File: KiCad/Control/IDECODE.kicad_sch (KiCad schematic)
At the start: 17 parts, among them U10 74HCT32, U12 28C16, U13 28C16, U14 74HCT163, U15 74HCT00, U16 74HCT32, U17 74HCT04, U2 74HCT04, U23 74HCT04, U28 74HCT08, U9 74HCT08

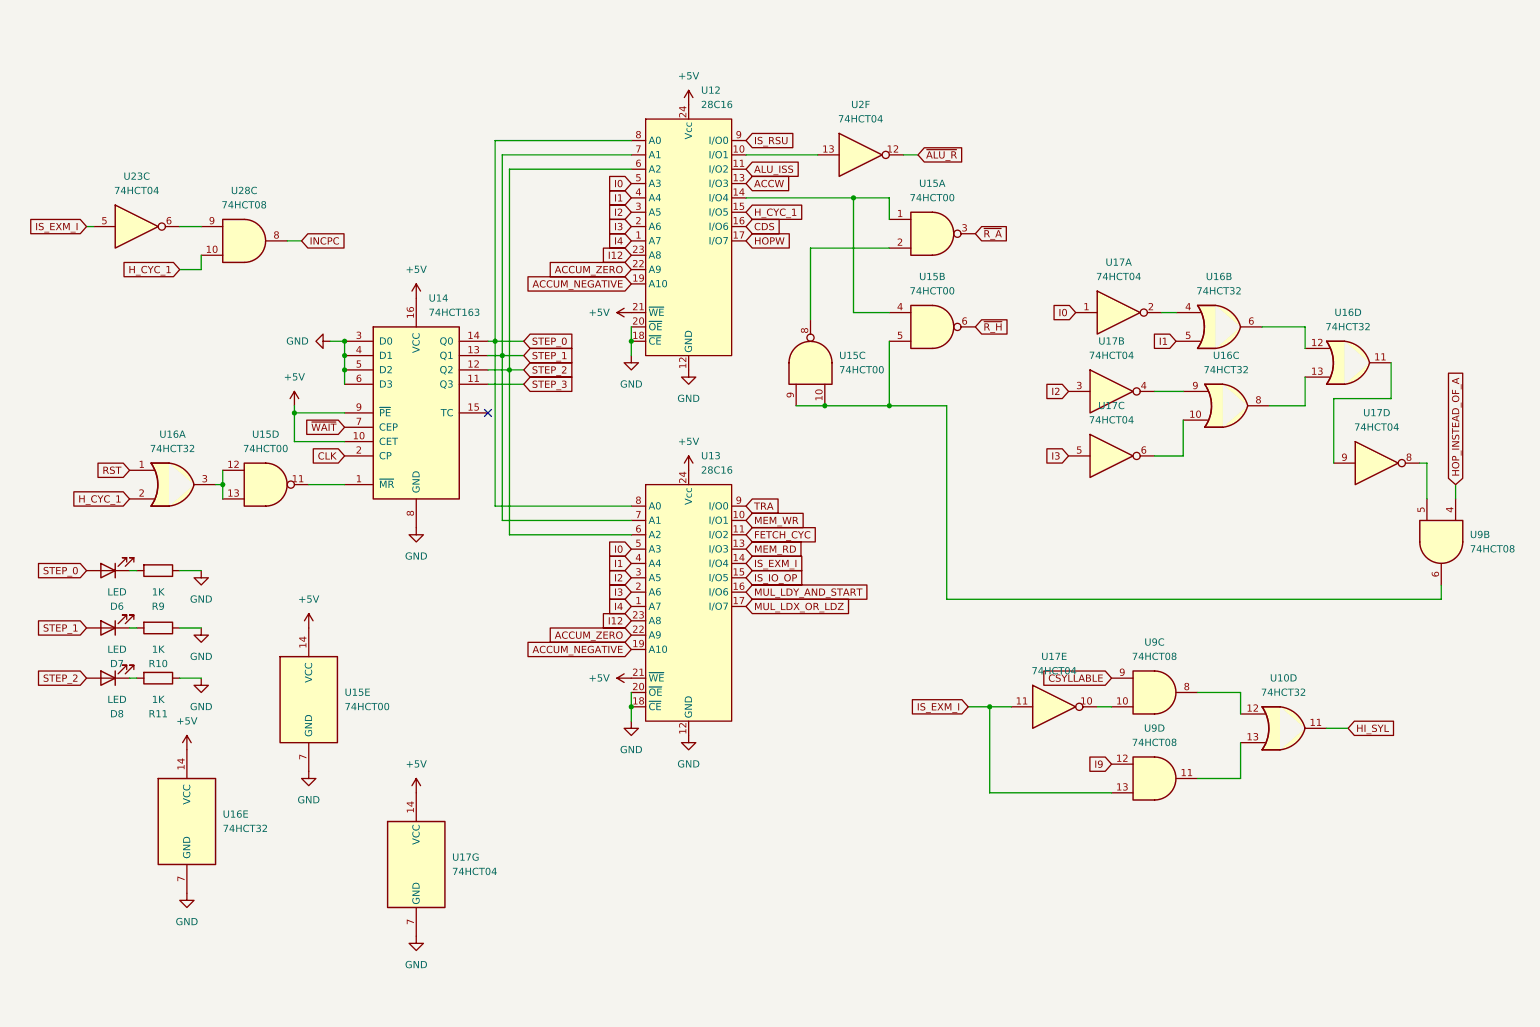
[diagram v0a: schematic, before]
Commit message: Update schematics with fixes.
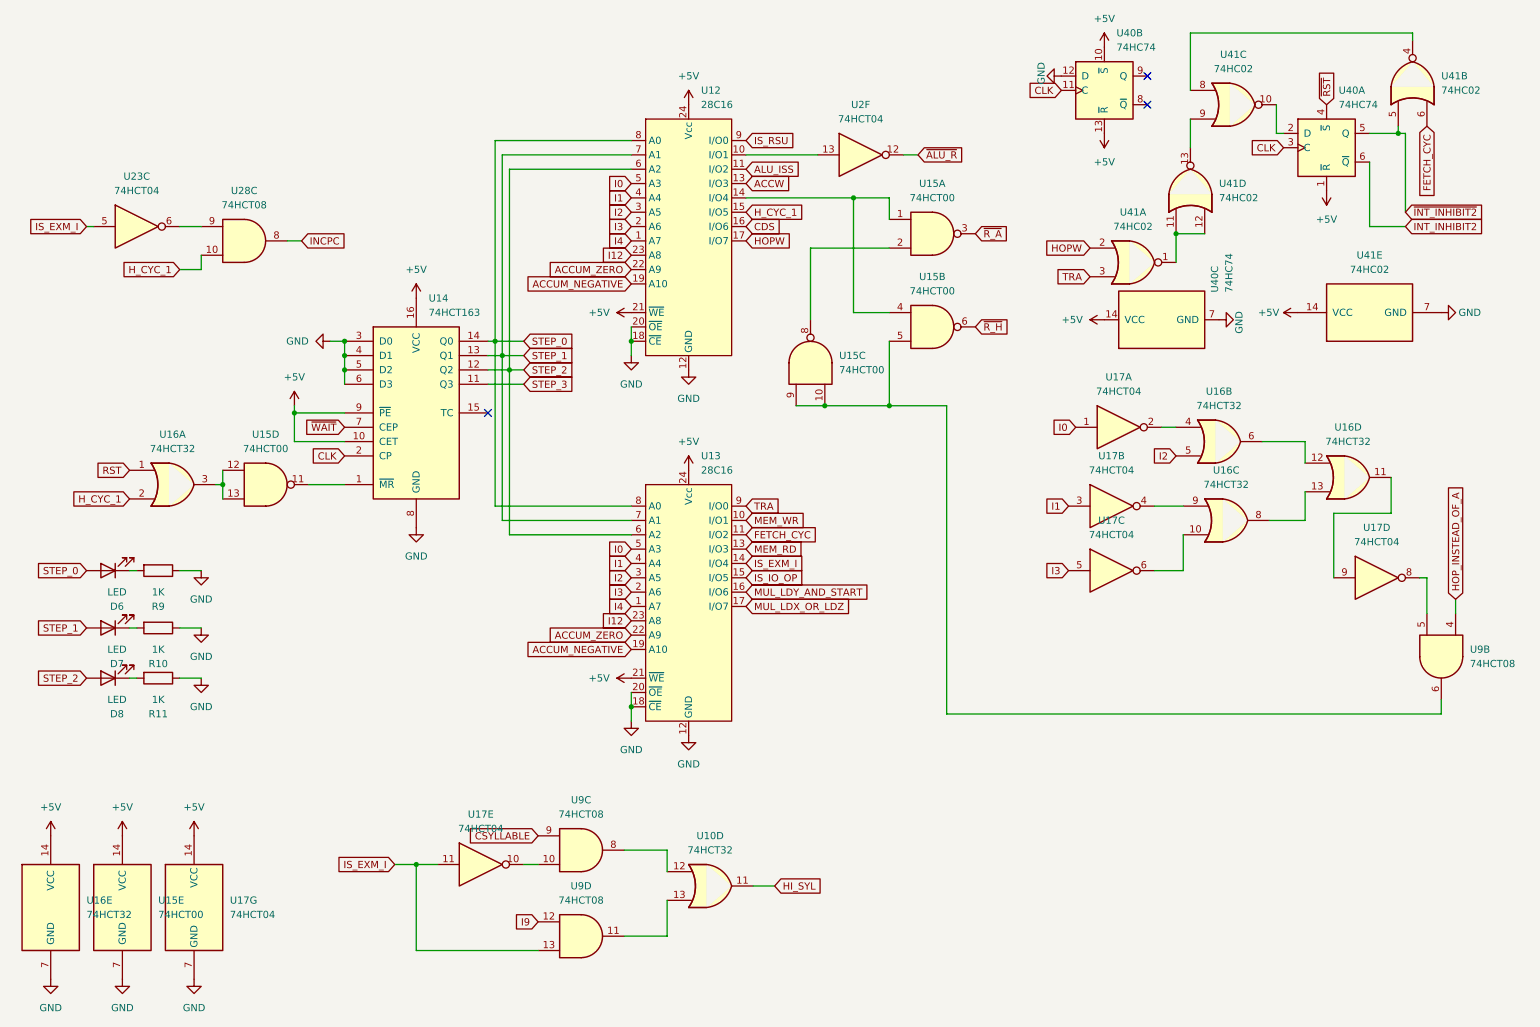
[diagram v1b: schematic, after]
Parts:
- added U40: 74HC74, Package_SO:SO-14_3.9x8.65mm_P1.27mm, symbol 74xx:74HC74
- added U41: 74HC02, Package_SO:SO-14_3.9x8.65mm_P1.27mm, symbol 74xx:74HC02
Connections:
- net +5V: now also U40.1 (~{R}), U40.10 (~{S}), U40.13 (~{R}), U40.14 (VCC), U41.14 (VCC)
- net CLK: now also U40.11 (C), U40.3 (C)
- net FETCH_CYC: now also U41.6
- net GND: now also U40.12 (D), U40.7 (GND), U41.7 (GND)
- net HOPW: now also U41.2
- net I1: now also U17.3; no longer U16.5
- net I2: now also U16.5; no longer U17.3
- net TRA: now also U41.3
- new net: U41.4, U41.8
- new net: U40.2 (D), U41.10
- new net: U41.1, U41.11, U41.12
- new net: U41.13, U41.9
- new net INT_INHIBIT2: U40.6 (~{Q})
- new net ~{INT_INHIBIT2}: U40.5 (Q), U41.5
- new net ~{RST}: U40.4 (~{S})
- no-connect marks 1 -> 3
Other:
- moved on the sheet: U10D, U15E, U16B, U16C, U16D, U16E, U17A, U17B, U17C, U17D, U17E, U17G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
